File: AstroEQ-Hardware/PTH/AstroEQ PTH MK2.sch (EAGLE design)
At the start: 40 parts, among them IC1 ATMEGA162-16PU, IC2 PIC18F14K50-I/P, IC3 78L05, J1 POWER_JACKPTH, M1 Motor Driver, M2 Motor Driver, X1 16MHz, X2 12MHz

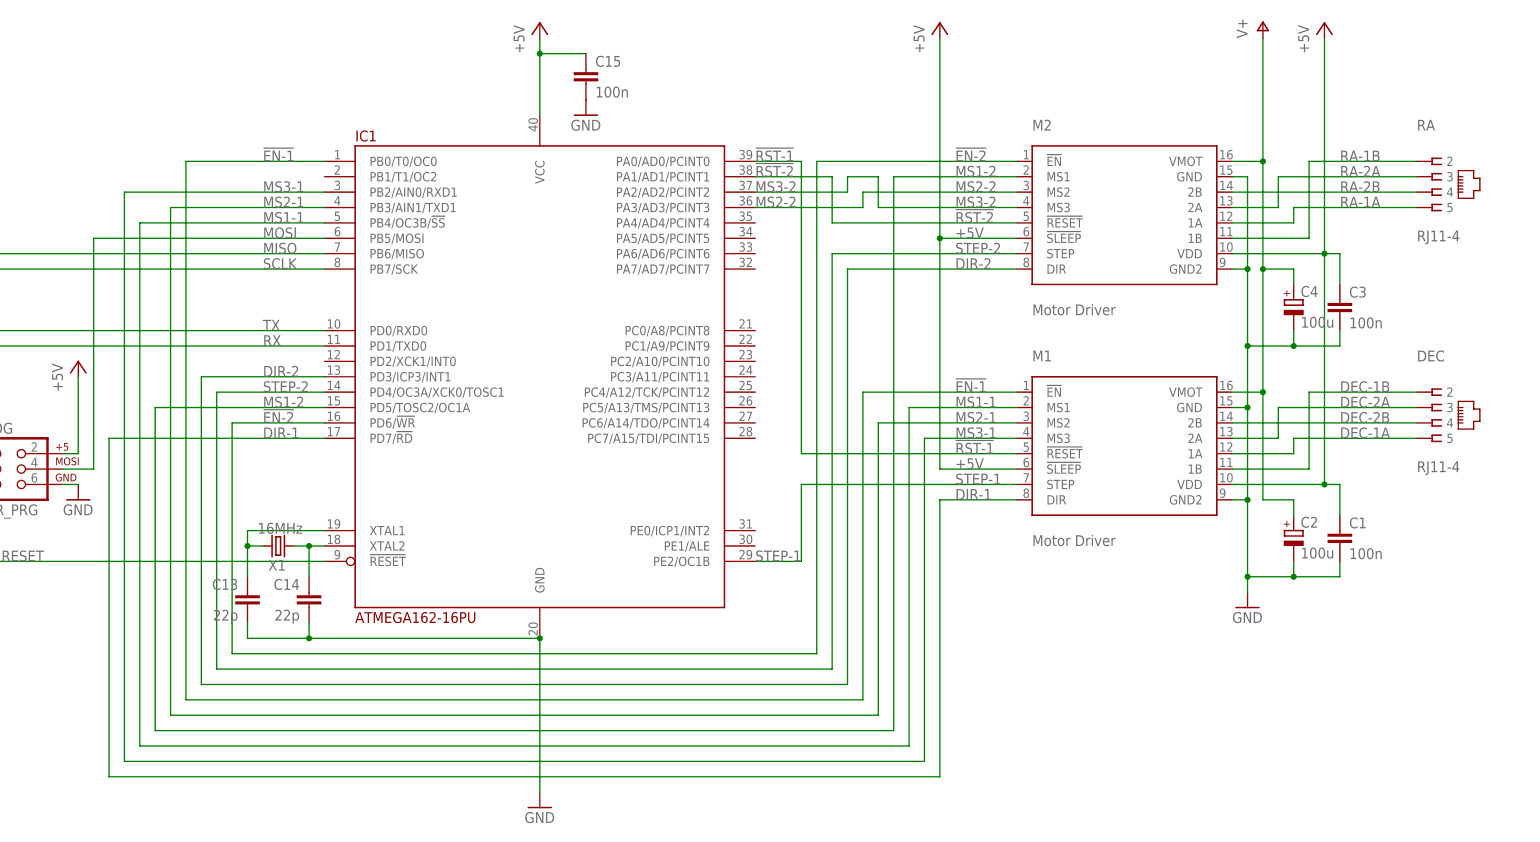
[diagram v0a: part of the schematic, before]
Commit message: New AstroEQ Version
AstroEQ6 has been released and is better than ever!
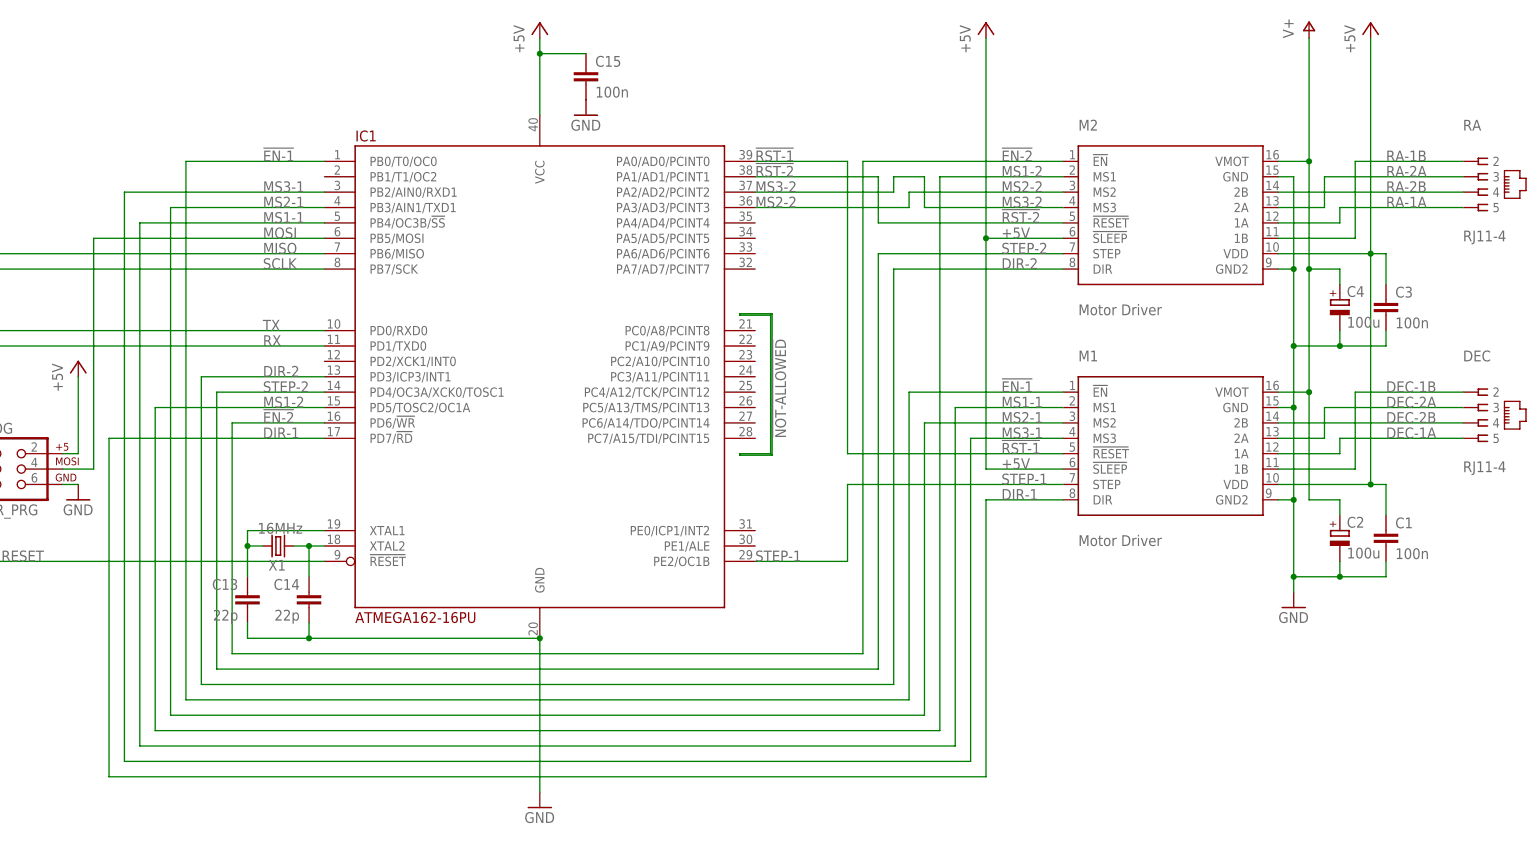
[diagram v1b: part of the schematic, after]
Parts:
- DEC, RA: MF (none) -> MOLEX; MPN (none) -> 95501-2641; OC_FARNELL (none) -> 1560166
- IC2: MPN PIC18F14K50-I/P -> (none); OC_FARNELL 1648501 -> (none)
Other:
- moved on the sheet: C1, C2, C3, C4, DEC, M1, M2, RA
